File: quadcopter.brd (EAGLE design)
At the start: 137.3 x 137.3 mm, 71 parts, among them J1 AVR_SPI_PRG_6NS, U1 ATMEGA128RFA1, Y2 16MHz

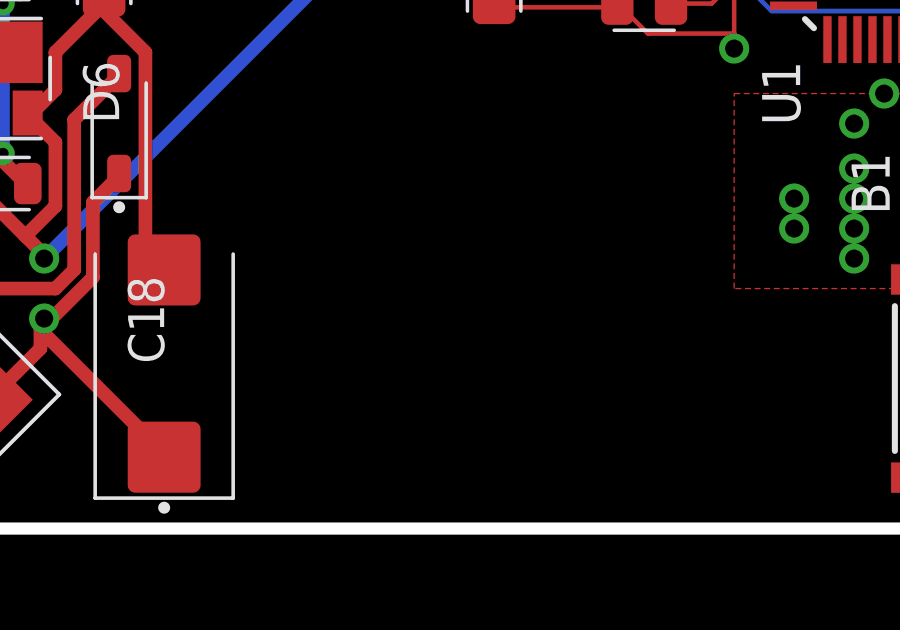
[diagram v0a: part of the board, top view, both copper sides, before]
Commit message: commiting new CAM files and new board logos
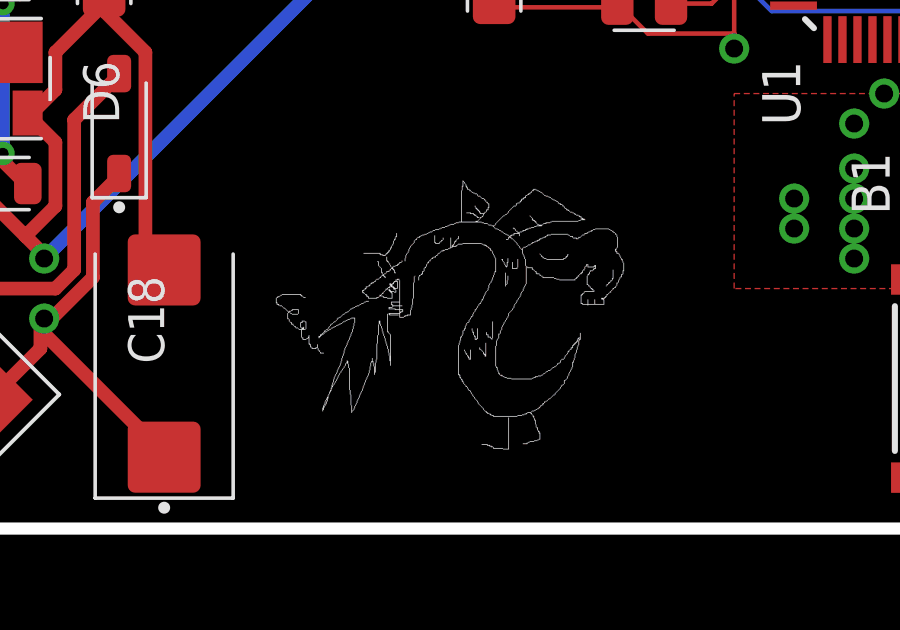
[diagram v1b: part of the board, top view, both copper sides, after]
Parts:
- added U$12: (no value), logos:TROGDOR
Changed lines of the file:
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@@
 <element name="U$10" library="logos" package="DERPY_BATMAN" value="" x="16" y="48"/>
 <element name="U$11" library="logos" package="MUFFIN_MAN" value="" x="39" y="45"/>
+<element name="U$12" library="logos" package="TROGDOR" value="" x="15" y="-2"/>
 </elements>
 <signals>
